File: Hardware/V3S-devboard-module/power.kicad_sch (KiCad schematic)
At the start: 68 parts, among them U101 EA3036C, U102 XC6206PxxxMR

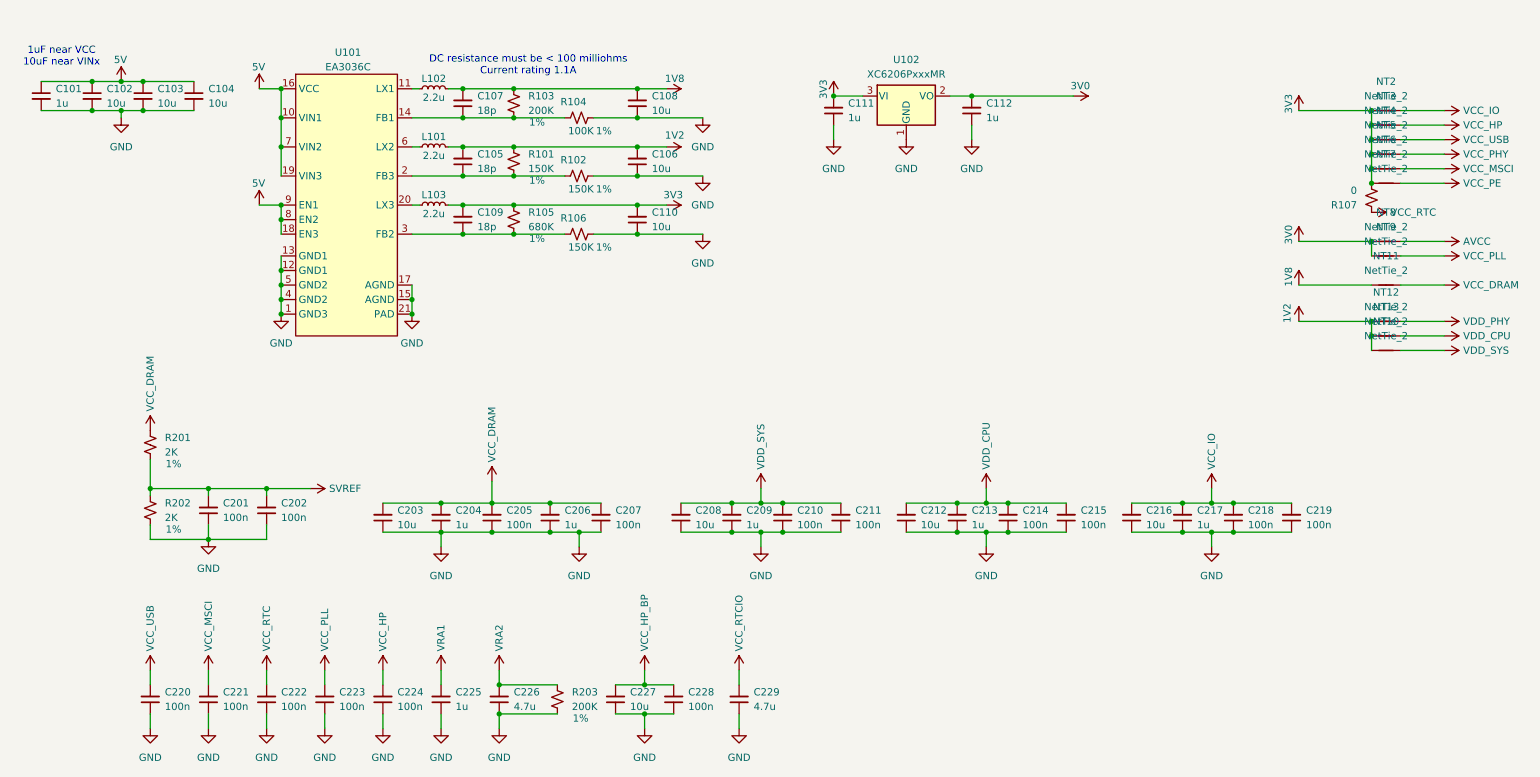
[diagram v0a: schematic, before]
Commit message: layout
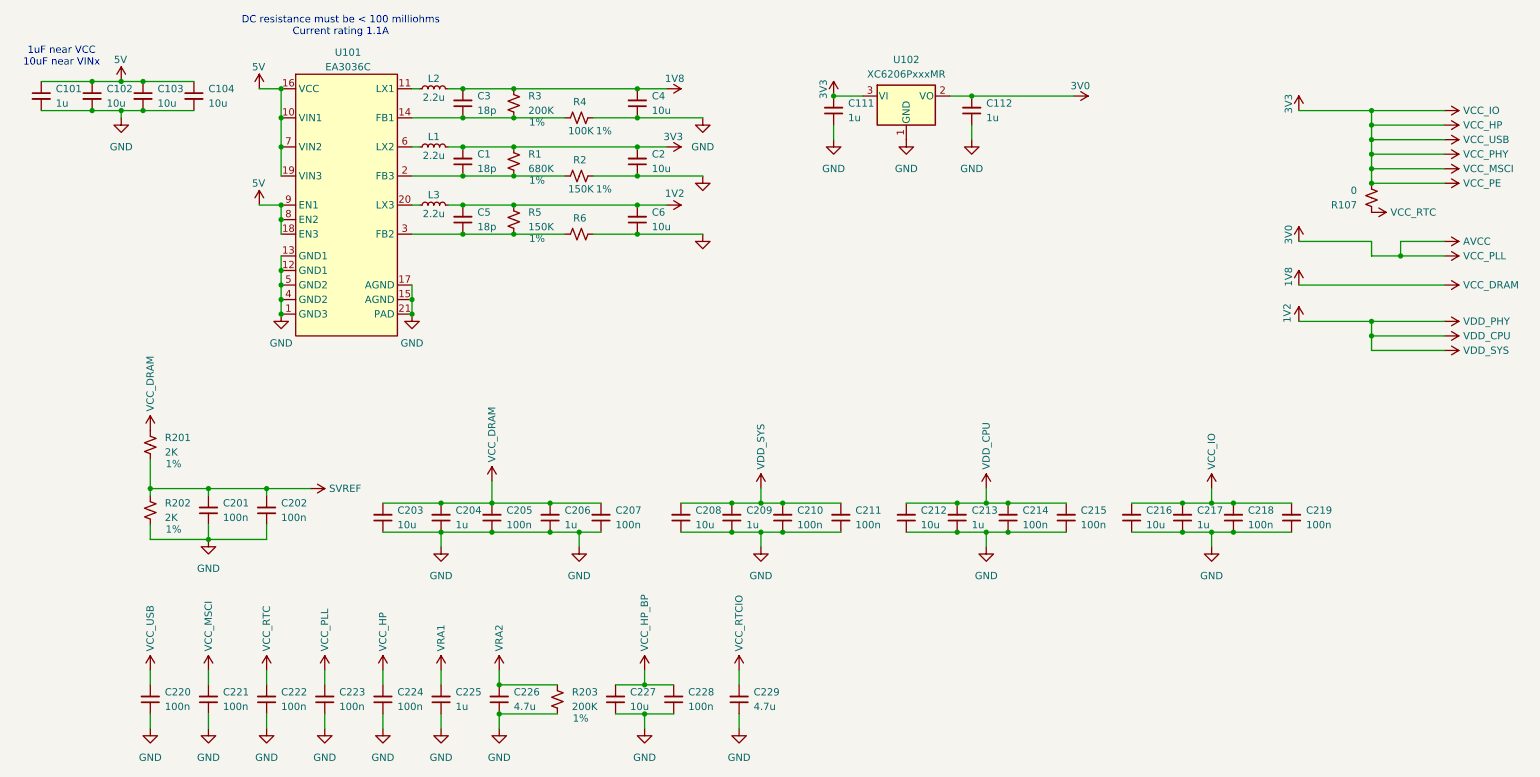
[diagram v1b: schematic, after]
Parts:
- removed C105, C107, C109: 18p, Capacitor_SMD:C_0402_1005Metric, symbol Device:C_Small
- removed C106, C108, C110: 10u, Capacitor_SMD:C_0603_1608Metric, symbol Device:C_Small
- removed L101, L102, L103: 2.2u, Inductor_SMD:L_1008_2520Metric, symbol Device:L_Small
- removed NT10, NT11, NT12, NT13, NT2, NT3, NT4, NT5, NT6, NT7, NT8, NT9: NetTie_2, NetTie:NetTie-2_SMD_Pad0.5mm, symbol Device:NetTie_2
- removed R101, R102, R106: 150K, Resistor_SMD:R_0402_1005Metric, symbol Device:R_Small_US
- removed R103: 200K, Resistor_SMD:R_0402_1005Metric, symbol Device:R_Small_US
- removed R104: 100K, Resistor_SMD:R_0402_1005Metric, symbol Device:R_Small_US
- removed R105: 680K, Resistor_SMD:R_0402_1005Metric, symbol Device:R_Small_US
- added C1, C3, C5: 18p, Capacitor_SMD:C_0402_1005Metric, symbol Device:C_Small
- added C2, C4, C6: 10u, Capacitor_SMD:C_0603_1608Metric, symbol Device:C_Small
- added L1, L2, L3: 2.2u, Inductor_SMD:L_1008_2520Metric, symbol Device:L_Small
- added R1: 680K, Resistor_SMD:R_0402_1005Metric, symbol Device:R_Small_US
- added R2, R5, R6: 150K, Resistor_SMD:R_0402_1005Metric, symbol Device:R_Small_US
- added R3: 200K, Resistor_SMD:R_0402_1005Metric, symbol Device:R_Small_US
- added R4: 100K, Resistor_SMD:R_0402_1005Metric, symbol Device:R_Small_US
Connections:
- net VCC_DRAM is gone; now on net 1V8: C203.2, C204.2, C205.2, C206.2, C207.2, R201.1
- net VCC_HP is gone; now on net 3V3: C224.2
- net VCC_IO is gone; now on net 3V3: C216.2, C217.2, C218.2, C219.2
- net VCC_MSCI is gone; now on net 3V3: C221.2
- net VCC_PLL is gone; now on net 3V0: C223.2
- net VCC_USB is gone; now on net 3V3: C220.2
- net VDD_CPU is gone; now on net 1V2: C212.2, C213.2, C214.2, C215.2
- net VDD_SYS is gone; now on net 1V2: C208.2, C209.2, C210.2, C211.2
- net 1V2: now also C5.2, C6.2, L3.2, R5.1
- net 1V8: now also C3.2, C4.2, L2.2, R3.1
- net 3V3: now also C1.2, C2.2, L1.2, R1.1
- net GND: now also C2.1, C4.1, C6.1, R2.2, R4.2, R6.2
- net at U101.6 (LX2): now also L1.1
- net at U101.3 (FB2): now also C5.1, R5.2, R6.1
- net at U101.11 (LX1): now also L2.1
- net at U101.14 (FB1): now also C3.1, R3.2, R4.1
- net at U101.20 (LX3): now also L3.1
- net at U101.2 (FB3): now also C1.1, R1.2, R2.1
